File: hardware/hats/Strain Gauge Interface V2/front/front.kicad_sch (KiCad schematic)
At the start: 75 parts, among them J1 Conn_01x14, U1 ADS1235IRHBT, U2 ADS1235IRHBT, U3 LMR50410YQDBVRQ1, U5 BD450, U6 BD433

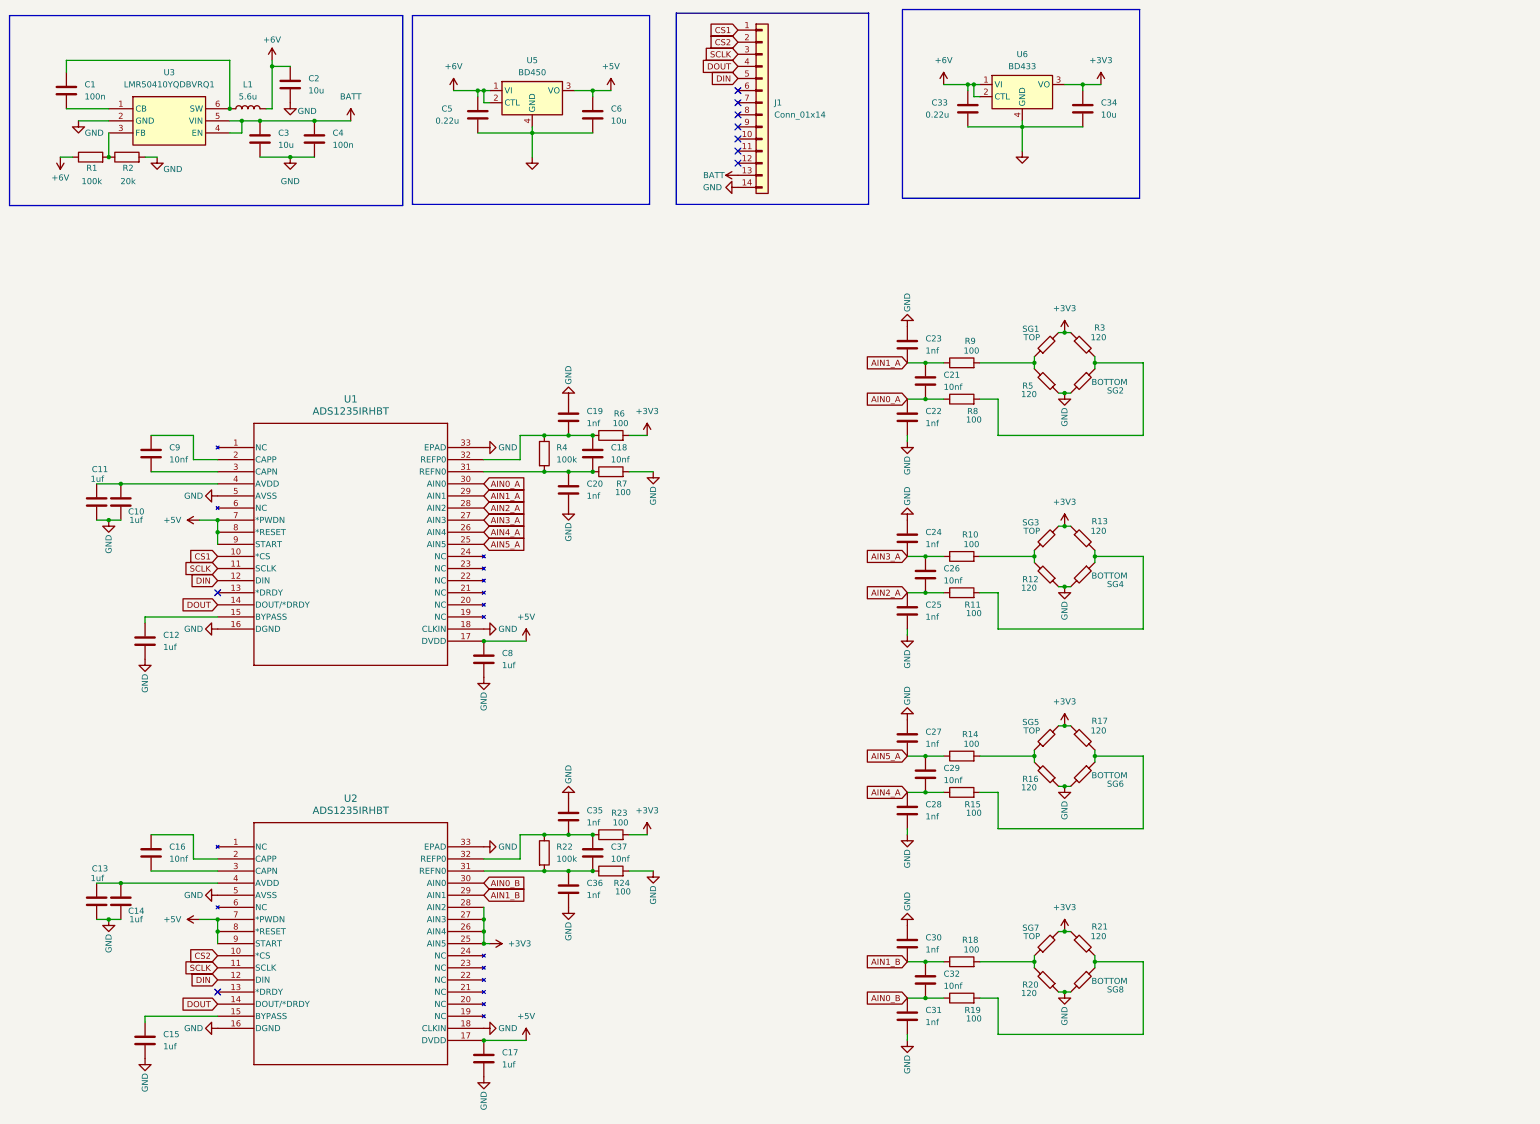
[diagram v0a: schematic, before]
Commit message: this is worse than torture
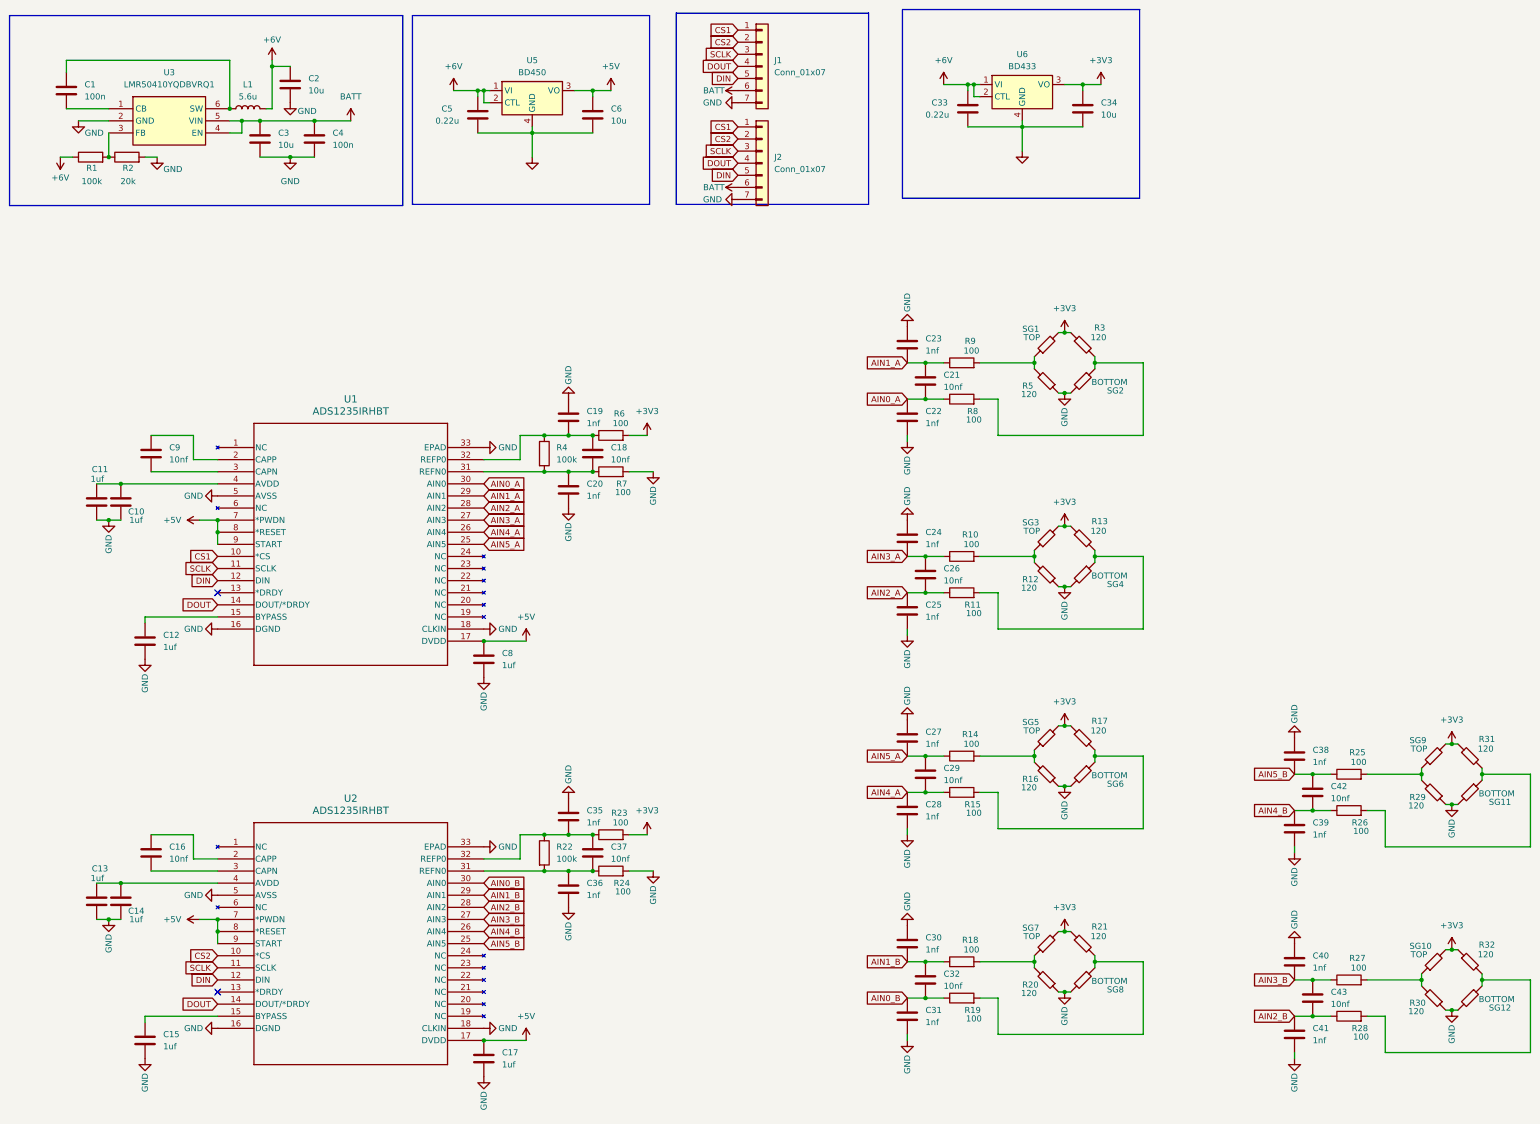
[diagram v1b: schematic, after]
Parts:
- removed J1: Conn_01x14, Connector_JST:JST_XA_S14B-XASK-1_1x14_P2.50mm_Horizontal, symbol Connector_Generic:Conn_01x14
- added C38, C39, C40, C41: 1nf, Capacitor_SMD:C_0603_1608Metric, symbol Device:C
- added C42, C43: 10nf, Capacitor_SMD:C_0603_1608Metric, symbol Device:C
- added J1, J2: Conn_01x07, Connector_JST:JST_XA_S07B-XASK-1_1x07_P2.50mm_Horizontal, symbol Connector_Generic:Conn_01x07
- added R25, R26, R27, R28: 100, Resistor_SMD:R_0603_1608Metric, symbol Device:R
- added R29, R30, R31, R32: 120, Resistor_SMD:R_0603_1608Metric, symbol Device:R_45deg
- added SG10, SG9: TOP, Connector_JST:JST_XA_S02B-XASK-1_1x02_P2.50mm_Horizontal, symbol Device:R_45deg
- added SG11, SG12: BOTTOM, Connector_JST:JST_XA_S02B-XASK-1_1x02_P2.50mm_Horizontal, symbol Device:R_45deg
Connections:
- net +3V3: now also R31.1, R32.1, SG10.2, SG9.2; no longer U2.25 (AIN5), U2.26 (AIN4), U2.27 (AIN3), U2.28 (AIN2)
- net BATT: now also J1.6 (Pin_6), J2.6 (Pin_6)
- net CS1: now also J1.1 (Pin_1), J2.1 (Pin_1)
- net CS2: now also J1.2 (Pin_2), J2.2 (Pin_2)
- net DIN: now also J1.5 (Pin_5), J2.5 (Pin_5)
- net DOUT: now also J1.4 (Pin_4), J2.4 (Pin_4)
- net GND: now also C38.1, C39.2, C40.1, C41.2, J1.7 (Pin_7), J2.7 (Pin_7), R29.1, R30.1, SG11.2, SG12.2
- net SCLK: now also J1.3 (Pin_3), J2.3 (Pin_3)
- new net: R28.2, R32.2, SG12.1
- new net: R25.2, R29.2, SG9.1
- new net: R27.2, R30.2, SG10.1
- new net: R26.2, R31.2, SG11.1
- new net AIN2_B: C41.1, C43.2, R28.1, U2.28 (AIN2)
- new net AIN3_B: C40.2, C43.1, R27.1, U2.27 (AIN3)
- new net AIN4_B: C39.1, C42.2, R26.1, U2.26 (AIN4)
- new net AIN5_B: C38.2, C42.1, R25.1, U2.25 (AIN5)
- no-connect marks 9 -> 2
